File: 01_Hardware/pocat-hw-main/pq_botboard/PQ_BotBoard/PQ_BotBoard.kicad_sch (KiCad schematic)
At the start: 37 parts, among them IC1 TCN75AVOA713, J1 53261-1471, J2 Conn_01x08_MountingPin, J5 Conn_01x03_MountingPin, U1 TPS7A7002DDAR

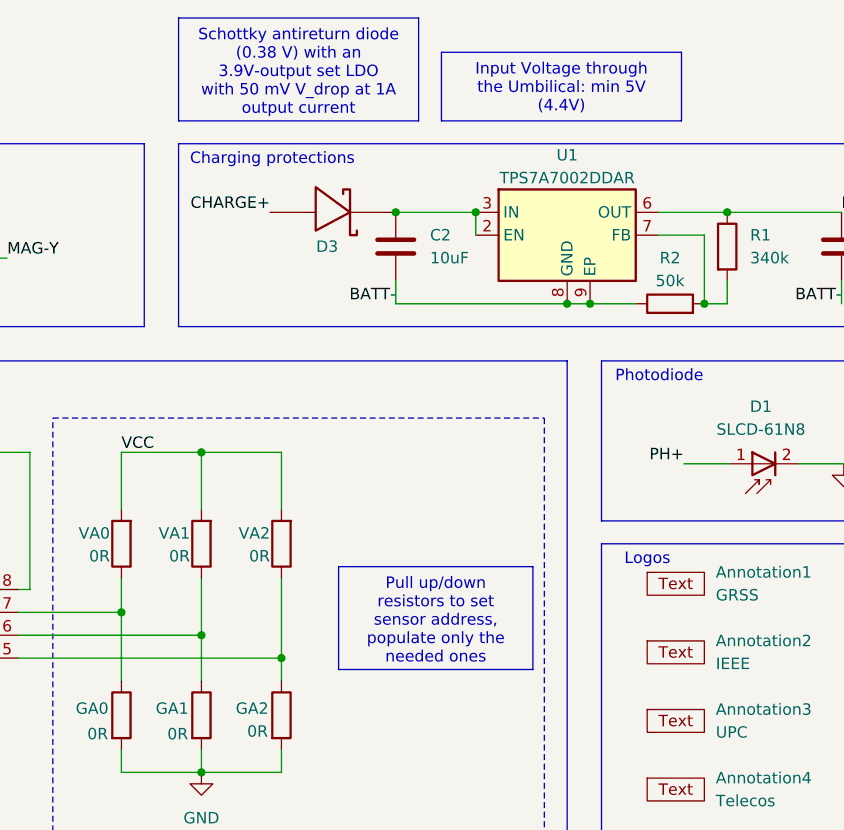
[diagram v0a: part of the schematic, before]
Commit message: Pcbs actualizados corregidos (son definitivos para mandarlos a fabricar con sus respectivos Gebers en una carpeta separada)
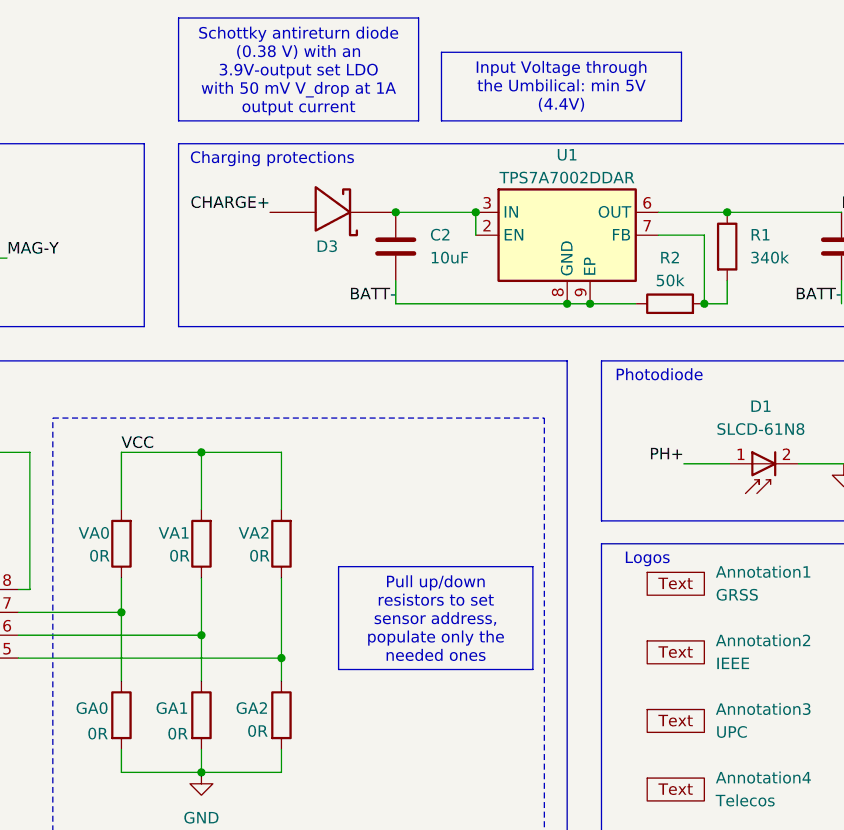
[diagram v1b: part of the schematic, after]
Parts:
- D3, SC2: value ~ -> (none)
- U1: value TPS7A7002DDAR -> TPS7A7002DDAR
